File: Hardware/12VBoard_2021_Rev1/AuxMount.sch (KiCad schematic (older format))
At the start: 33 parts, among them Q3 IRLML2060, Q4 CSD18537NQ5A, Q5 CSD18531Q5A, U1 LT1910, U10 LM5116, U11 INA198

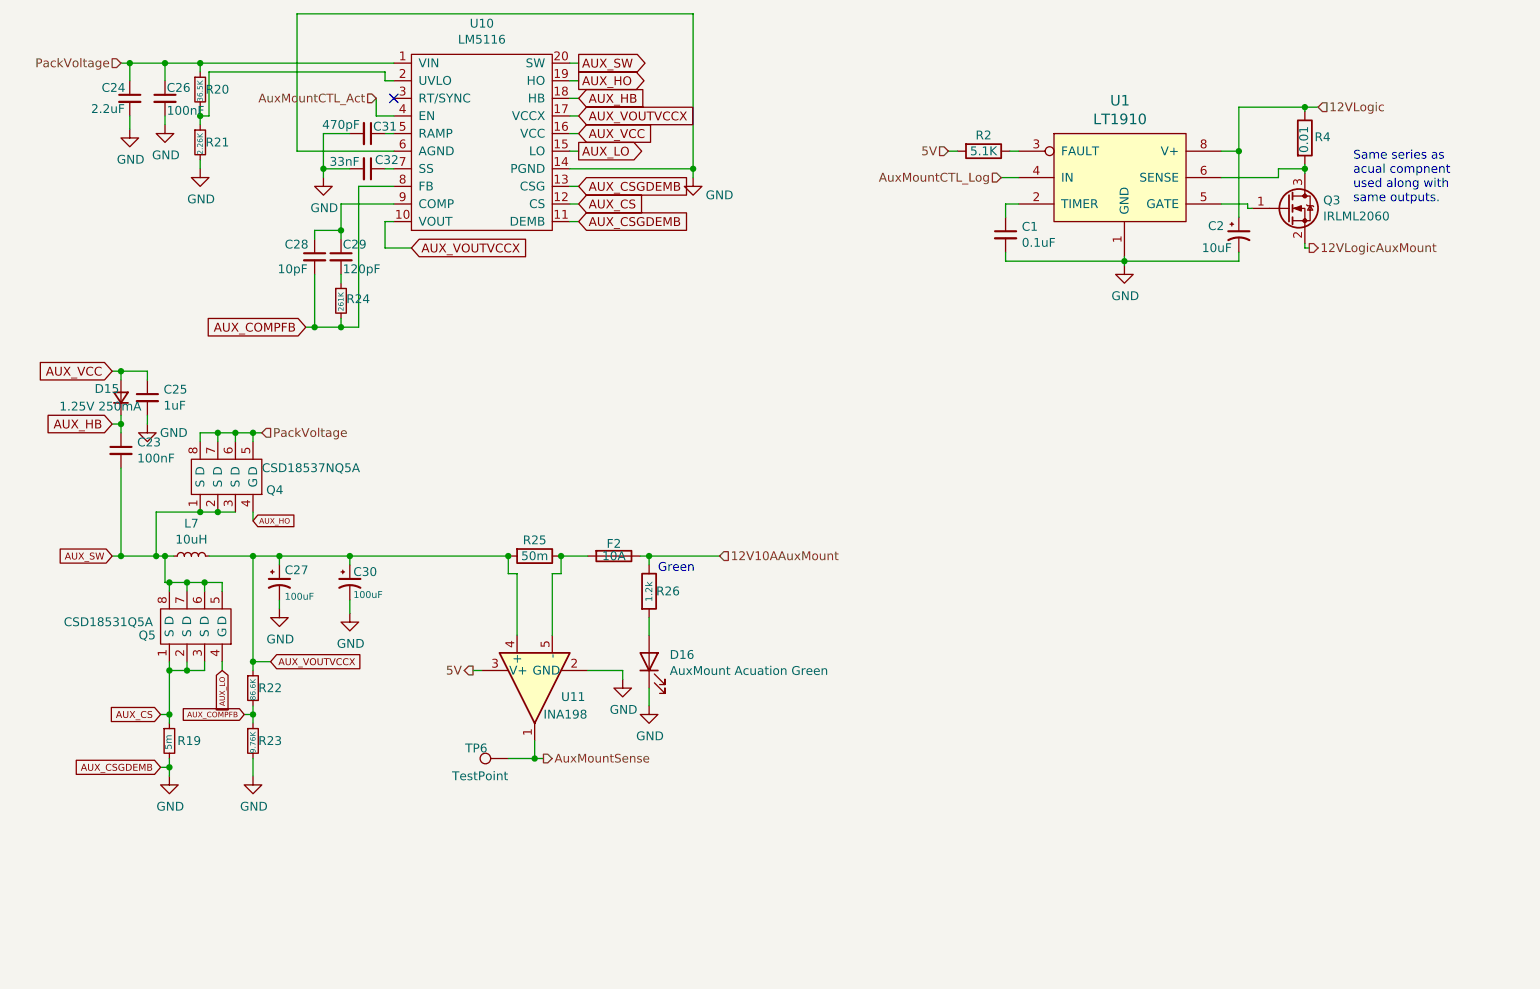
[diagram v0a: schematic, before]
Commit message: Started work on updated layout
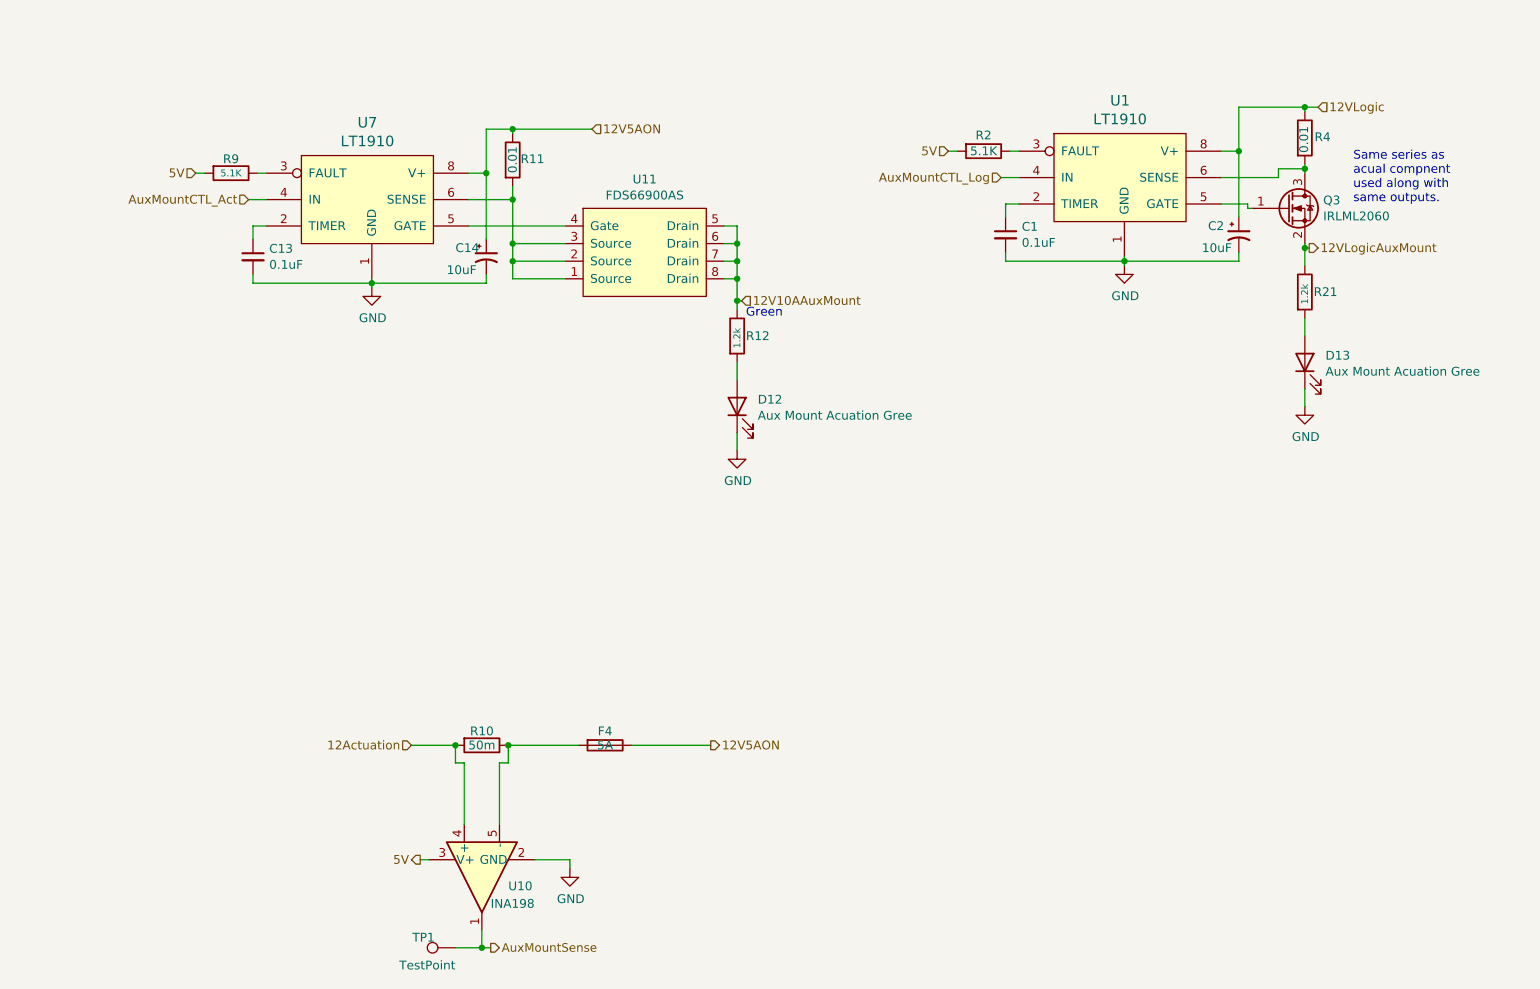
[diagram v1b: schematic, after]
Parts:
- removed C23, C26: 100nF, Capacitor_SMD:C_0603_1608Metric_Pad1.05x0.95mm_HandSolder, symbol Device:C_Small
- removed C24: 2.2uF, Capacitor_SMD:C_0603_1608Metric_Pad1.05x0.95mm_HandSolder, symbol Device:C_Small
- removed C25: 1uF, Capacitor_SMD:C_0603_1608Metric_Pad1.05x0.95mm_HandSolder, symbol Device:C_Small
- removed C27, C30: 100uF, Capacitor_THT:CP_Radial_D6.3mm_P2.50mm, symbol Device:CP1_Small
- removed C28: 10pF, Capacitor_SMD:C_0603_1608Metric_Pad1.05x0.95mm_HandSolder, symbol Device:C_Small
- removed C29: 120pF, Capacitor_SMD:C_0603_1608Metric_Pad1.05x0.95mm_HandSolder, symbol Device:C_Small
- removed C31: 470pF, Capacitor_SMD:C_0603_1608Metric_Pad1.05x0.95mm_HandSolder, symbol Device:C_Small
- removed C32: 33nF, Capacitor_SMD:C_0603_1608Metric_Pad1.05x0.95mm_HandSolder, symbol Device:C_Small
- removed D15: 1.25V 250mA, Diode_SMD:D_SOD-323_HandSoldering, symbol Device:D_Small
- removed D16: AuxMount Acuation Green, Diode_SMD:D_0603_1608Metric_Pad1.05x0.95mm_HandSolder, symbol Device:LED
- removed F2: 10A, MRDT_Passives:ATC_Fuse_Block, symbol Device:Fuse
- removed L7: 10uH, Inductor_THT:L_Radial_D27.9mm_P20.07mm_Vishay_IHB-3, symbol Device:L_Small
- removed Q4: CSD18537NQ5A, Package_SON:VSONP-8-1EP_5x6_P1.27mm, symbol 12VBoard_2021_Rev1-rescue:CSD18537NQ5A
- removed Q5: CSD18531Q5A, Package_SON:VSONP-8-1EP_5x6_P1.27mm, symbol 12VBoard_2021_Rev1-rescue:CSD18531Q5A
- removed R19: 5m, Resistor_SMD:R_0603_1608Metric_Pad1.05x0.95mm_HandSolder, symbol Device:R_Small
- removed R20: 36.5K, Resistor_SMD:R_0603_1608Metric_Pad1.05x0.95mm_HandSolder, symbol Device:R_Small
- removed R21: 2.26K, Resistor_SMD:R_0603_1608Metric_Pad1.05x0.95mm_HandSolder, symbol Device:R_Small
- removed R22: 86.6K, Resistor_SMD:R_0603_1608Metric_Pad1.05x0.95mm_HandSolder, symbol Device:R_Small
- removed R23: 9.76K, Resistor_SMD:R_0603_1608Metric_Pad1.05x0.95mm_HandSolder, symbol Device:R_Small
- removed R24: 261K, Resistor_SMD:R_0603_1608Metric_Pad1.05x0.95mm_HandSolder, symbol Device:R_Small
- removed R25: 50m, Package_TO_SOT_THT:TO-126-2_Vertical, symbol Device:R
- removed R26: 1.2k, Resistor_SMD:R_0603_1608Metric_Pad1.05x0.95mm_HandSolder, symbol Device:R
- removed TP6: TestPoint, TestPoint:TestPoint_Pad_2.5x2.5mm, symbol Connector:TestPoint
- removed U10: LM5116, Package_SO:TSSOP-20_4.4x6.5mm_P0.65mm, symbol 12VBoard_2021_Rev1-rescue:LM5116
- removed U11: INA198, Package_TO_SOT_SMD:SOT-23-5, symbol Amplifier_Current:INA198
- added C13: 0.1uF, Capacitor_SMD:C_0603_1608Metric_Pad1.05x0.95mm_HandSolder, symbol Device:C_Small
- added C14: 10uF, Capacitor_THT:CP_Radial_D5.0mm_P2.00mm, symbol Device:CP1_Small
- added D12, D13: Aux Mount Acuation Gree, Diode_SMD:D_0603_1608Metric_Pad1.05x0.95mm_HandSolder, symbol Device:LED
- added F4: 5A, MRDT_Passives:ATC_Fuse_Block, symbol Device:Fuse
- added R10: 50m, Package_TO_SOT_THT:TO-126-2_Vertical, symbol Device:R
- added R11: 0.01, Resistor_SMD:R_0603_1608Metric_Pad1.05x0.95mm_HandSolder, symbol Device:R
- added R12, R21: 1.2k, Resistor_SMD:R_0603_1608Metric_Pad1.05x0.95mm_HandSolder, symbol Device:R
- added R9: 5.1K, Resistor_SMD:R_0603_1608Metric_Pad1.05x0.95mm_HandSolder, symbol Device:R
- added TP1: TestPoint, TestPoint:TestPoint_Pad_2.5x2.5mm, symbol Connector:TestPoint
- added U10: INA198, Package_TO_SOT_SMD:SOT-23-5, symbol Amplifier_Current:INA198
- added U11: FDS66900AS, Package_SO:SOIC-8_3.9x4.9mm_P1.27mm, symbol 12VBoard_2021_Rev1:FDS66900AS
- added U7: LT1910, Package_SO:SOIC-8-N7_3.9x4.9mm_P1.27mm, symbol MRDT_ICs:LT1910
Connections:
- net 12V10AAuxMount: now also R12.1, U11.5 (Drain), U11.6 (Drain), U11.7 (Drain), U11.8 (Drain)
- net 12VLogicAuxMount: now also R21.1
- net 5V: now also R9.2, U10.3 (V+)
- net AuxMountCTL_Act: now also U7.4 (IN)
- net AuxMountSense: now also TP1.1, U10.1
- net GND: now also C13.2, C14.2, D12.1 (K), D13.1 (K), U10.2 (GND), U7.1 (GND)
- new net: D12.2 (A), R12.2
- new net: F4.2, R10.1, U10.5 (-)
- new net: C13.1, U7.2 (TIMER)
- new net: R9.1, U7.3 (FAULT)
- new net: U11.4 (Gate), U7.5 (GATE)
- new net: R11.2, U11.1 (Source), U11.2 (Source), U11.3 (Source), U7.6 (SENSE)
- new net: D13.2 (A), R21.2
- new net 12Actuation: R10.2, U10.4 (+)
- new net 12V5AON: C14.1, F4.1, R11.1, U7.8 (V+)
- no-connect marks 1 -> 0
